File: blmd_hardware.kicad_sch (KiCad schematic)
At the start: 63 parts, among them J1 MR30PW-F, J2 control, J3 GND, J4 12V, J5 STLink-V3, Q1 RH6G040CH, Q2 RH6G040CH, Q3 RH6G040CH, Q4 RH6G040CH, Q5 RH6G040CH, Q6 RH6G040CH, SW1 reset, SW2 SW_DIP_x02, U1 A4939KLPTR-5-T, U10 STM32G431KBTx, U4 ISO7760FDBQR, U6 ACS711KEXLT-31AB, U7 ACS711KEXLT-31AB, U9 BD41041FJ-C

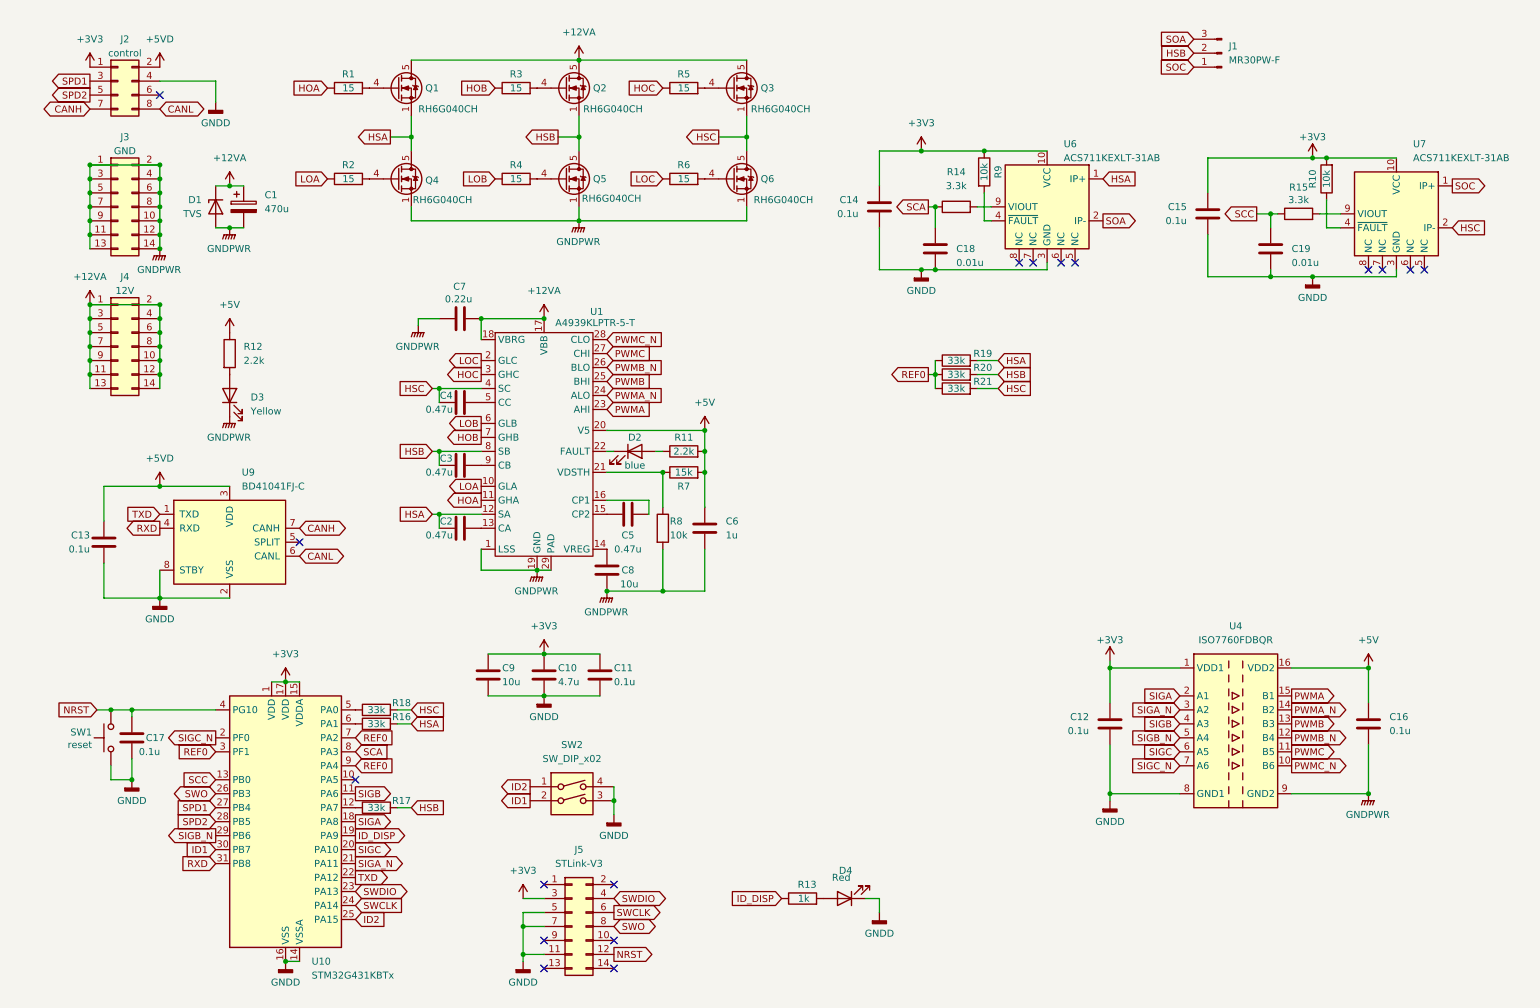
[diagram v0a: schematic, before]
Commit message: tmp : schemetic is all over except for can
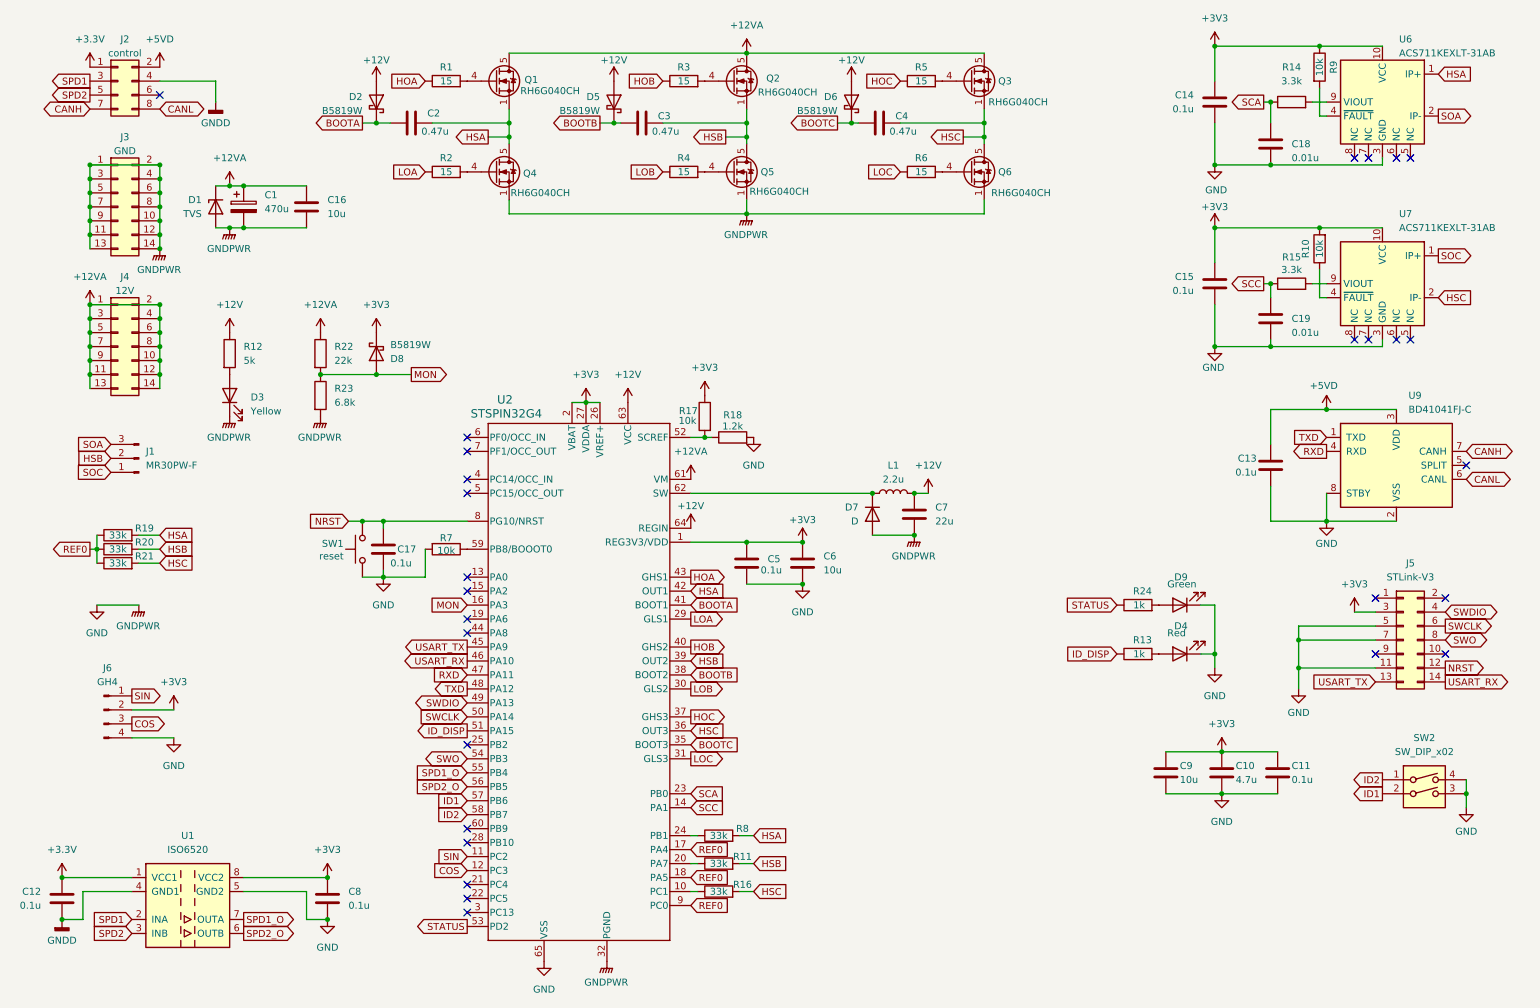
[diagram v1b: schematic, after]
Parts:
- removed D2: blue, LED_SMD:LED_0603_1608Metric_Pad1.05x0.95mm_HandSolder, symbol Device:LED
- removed U1: A4939KLPTR-5-T, Package_SO:HTSSOP-28-1EP_4.4x9.7mm_P0.65mm_EP2.75x6.2mm, symbol blmd:A4939KLPTR-5-T
- removed U10: STM32G431KBTx, Package_QFP:LQFP-32_7x7mm_P0.8mm, symbol MCU_ST_STM32G4:STM32G431KBTx
- removed U4: ISO7760FDBQR, Package_SO:SSOP-16_3.9x4.9mm_P0.635mm, symbol Isolator:Si8660BA-AS1
- added D2, D5, D6, D8: B5819W, Diode_SMD:D_SOD-123, symbol Device:D_Schottky
- added D7: D, symbol Device:D
- added D9: Green, LED_SMD:LED_0603_1608Metric_Pad1.05x0.95mm_HandSolder, symbol Device:LED
- added J6: GH4, symbol Connector:Conn_01x04_Pin
- added L1: 2.2u, symbol Device:L
- added R22: 22k, symbol Device:R
- added R23: 6.8k, symbol Device:R
- added R24: 1k, Resistor_SMD:R_0603_1608Metric_Pad0.98x0.95mm_HandSolder, symbol Device:R
- added U1: ISO6520, Package_SO:SOIC-8_3.9x4.9mm_P1.27mm, symbol Isolator:ISO7320C
- added U2: STSPIN32G4, QFN_IN32G4_STM, symbol blmd:STSPIN32G4
- C12, C2, C3, C4: footprint Capacitor_SMD:C_0603_1608Metric_Pad1.08x0.95mm_HandSolder -> (none)
- C16: value 0.1u -> 10u; footprint Capacitor_SMD:C_0603_1608Metric_Pad1.08x0.95mm_HandSolder -> (none)
- C5: value 0.47u -> 0.1u; footprint Capacitor_SMD:C_0603_1608Metric_Pad1.08x0.95mm_HandSolder -> (none)
- C6: value 1u -> 10u; footprint Capacitor_SMD:C_0603_1608Metric_Pad1.08x0.95mm_HandSolder -> (none)
- C7: value 0.22u -> 22u; footprint Capacitor_SMD:C_0603_1608Metric_Pad1.08x0.95mm_HandSolder -> (none)
- C8: value 10u -> 0.1u; footprint Capacitor_SMD:C_0603_1608Metric_Pad1.08x0.95mm_HandSolder -> (none)
- R11: value 2.2k -> 33k; footprint Resistor_SMD:R_0603_1608Metric_Pad0.98x0.95mm_HandSolder -> (none)
- R12: value 2.2k -> 5k
- R16: footprint Resistor_SMD:R_0603_1608Metric_Pad0.98x0.95mm_HandSolder -> (none)
- R17: value 33k -> 10k; footprint Resistor_SMD:R_0603_1608Metric_Pad0.98x0.95mm_HandSolder -> (none)
- R18: value 33k -> 1.2k; footprint Resistor_SMD:R_0603_1608Metric_Pad0.98x0.95mm_HandSolder -> (none)
- R7: value 15k -> 10k; footprint Resistor_SMD:R_0603_1608Metric_Pad0.98x0.95mm_HandSolder -> (none)
- R8: value 10k -> 33k; footprint Resistor_SMD:R_0603_1608Metric_Pad0.98x0.95mm_HandSolder -> (none)
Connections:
- net +12VA: now also C16.1, R22.1, U2.61 (VM); no longer C7.1
- net +3V3: now also C5.1, C6.1, C8.1, R17.1, D8.1 (K), J6.2 (Pin_2), U1.8 (VCC2), U2.1 (REG3V3/VDD), U2.2 (VBAT), U2.26 (VREF+), U2.27 (VDDA); no longer C12.1, J2.1 (Pin_1)
- net GNDD: now also U1.4 (GND1); no longer C10.2, C11.2, C13.2, C14.2, C15.2, C17.2, C18.2, C19.2, C9.2, D4.1 (K), J5.11 (Pin_11), J5.5 (Pin_5), J5.7 (Pin_7), SW1.1, SW2.3, SW2.4, U6.3 (GND), U7.3 (GND), U9.2 (VSS), U9.8 (STBY)
- net HOA: now also U2.43 (GHS1)
- net HOB: now also U2.40 (GHS2)
- net HOC: now also U2.37 (GHS3)
- net HSA: now also R8.2, U2.42 (OUT1); no longer R16.2
- net HSB: now also C3.2, R11.2, U2.39 (OUT2); no longer C3.1, R17.2
- net HSC: now also C4.2, R16.2, U2.36 (OUT3); no longer C4.1, R18.2
- net ID1: now also U2.57 (PB6)
- net ID2: now also U2.58 (PB7)
- net ID_DISP: now also U2.51 (PA15)
- net LOA: now also U2.29 (GLS1)
- net LOB: now also U2.30 (GLS2)
- net LOC: now also U2.31 (GLS3)
- net NRST: now also U2.8 (PG10/NRST)
- net REF0: now also U2.17 (PA4), U2.18 (PA5), U2.9 (PC0)
- net RXD: now also U2.47 (PA11)
- net SCA: now also U2.23 (PB0)
- net SCC: now also U2.14 (PA1)
- net SPD1: now also U1.2 (INA)
- net SPD2: now also U1.3 (INB)
- net SWCLK: now also U2.50 (PA14)
- net SWDIO: now also U2.49 (PA13)
- net SWO: now also U2.54 (PB3)
- net TXD: now also U2.48 (PA12)
- net at R18.1: now also R17.2, U2.52 (SCREF)
- net at R16.1: now also U2.10 (PC1)
- net GND: now reaches C8.2
- net GND: now also C1.2, C10.2, C11.2, C13.2, C14.2, C15.2, C16.2, C17.2, C18.2, C19.2, C5.2, C6.2, C7.2, C9.2, D1.2 (A), D3.1 (K), D4.1 (K), J3.1 (Pin_1), J3.10 (Pin_10), J3.11 (Pin_11), J3.12 (Pin_12), J3.13 (Pin_13), J3.14 (Pin_14), J3.2 (Pin_2), J3.3 (Pin_3), J3.4 (Pin_4), J3.5 (Pin_5), J3.6 (Pin_6), J3.7 (Pin_7), J3.8 (Pin_8), J3.9 (Pin_9), J5.11 (Pin_11), J5.5 (Pin_5), J5.7 (Pin_7), Q4.1 (S), Q4.2 (S), Q4.3 (S), Q5.1 (S), Q5.2 (S), Q5.3 (S), Q6.1 (S), Q6.2 (S), Q6.3 (S), R18.2, R7.2, SW1.1, SW2.3, SW2.4, U6.3 (GND), U7.3 (GND), U9.2 (VSS), U9.8 (STBY), D7.2 (A), D9.1 (K), J6.4 (Pin_4), R23.2, U1.5 (GND2), U2.32 (PGND), U2.65 (VSS)
- net BOOTA: now reaches C2.2
- net BOOTA: now also D2.1 (K), U2.41 (BOOT1)
- net at R8.1: now also U2.24 (PB1); no longer R7.1
- net at R11.1: now also U2.20 (PA7)
- net USART_TX: now reaches J5.13 (Pin_13)
- net USART_TX: now also U2.45 (PA9)
- net USART_RX: now reaches J5.14 (Pin_14)
- net USART_RX: now also U2.46 (PA10)
- removed net +5V: C16.1, C6.1, R11.2, R12.1, R7.2
- removed net GNDPWR: C1.2, C16.2, C6.2, C7.2, C8.1, D1.2 (A), D3.1 (K), J3.1 (Pin_1), J3.10 (Pin_10), J3.11 (Pin_11), J3.12 (Pin_12), J3.13 (Pin_13), J3.14 (Pin_14), J3.2 (Pin_2), J3.3 (Pin_3), J3.4 (Pin_4), J3.5 (Pin_5), J3.6 (Pin_6), J3.7 (Pin_7), J3.8 (Pin_8), J3.9 (Pin_9), Q4.1 (S), Q4.2 (S), Q4.3 (S), Q5.1 (S), Q5.2 (S), Q5.3 (S), Q6.1 (S), Q6.2 (S), Q6.3 (S), R8.2
- new net: D9.2 (A), R24.2
- new net: D7.1 (K), L1.1, U2.62 (SW)
- new net: U2.33 (NC), U2.34 (NC)
- new net: R7.1, U2.59 (PB8/BOOOT0)
- new net +12V: C7.1, D2.2 (A), D5.2 (A), D6.2 (A), L1.2, R12.1, U2.63 (VCC), U2.64 (REGIN)
- new net +3.3V: C12.1, J2.1 (Pin_1), U1.1 (VCC1)
- new net BOOTB: C3.1, D5.1 (K), U2.38 (BOOT2)
- new net BOOTC: C4.1, D6.1 (K), U2.35 (BOOT3)
- new net COS: J6.3 (Pin_3), U2.12 (PC3)
- new net MON: D8.2 (A), R22.2, R23.1, U2.16 (PA3)
- new net SIN: J6.1 (Pin_1), U2.11 (PC2)
- new net SPD1_O: U1.7 (OUTA), U2.55 (PB4)
- new net SPD2_O: U1.6 (OUTB), U2.56 (PB5)
- new net STATUS: R24.1, U2.53 (PD2)
- no-connect marks 17 -> 28
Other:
- moved on the sheet: C10, C11, C13, C14, C15, C17, C18, C19, C9, D4, J1, J5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

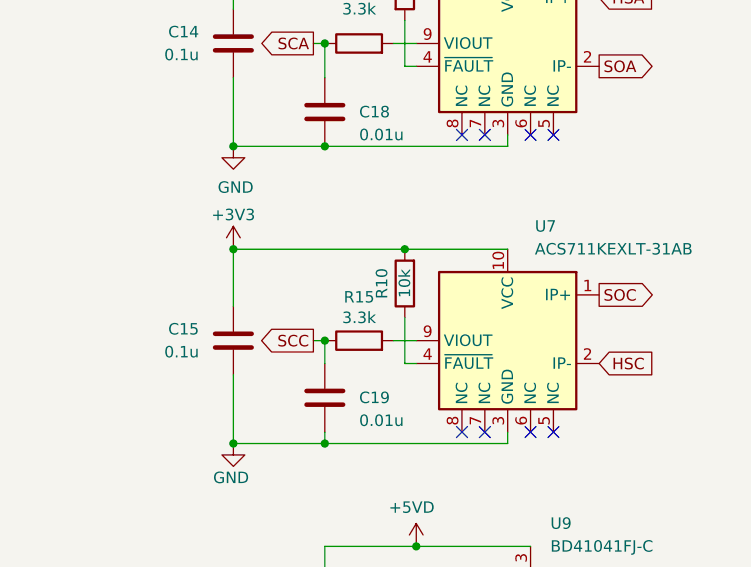
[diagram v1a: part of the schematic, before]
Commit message: tmp : backup commit
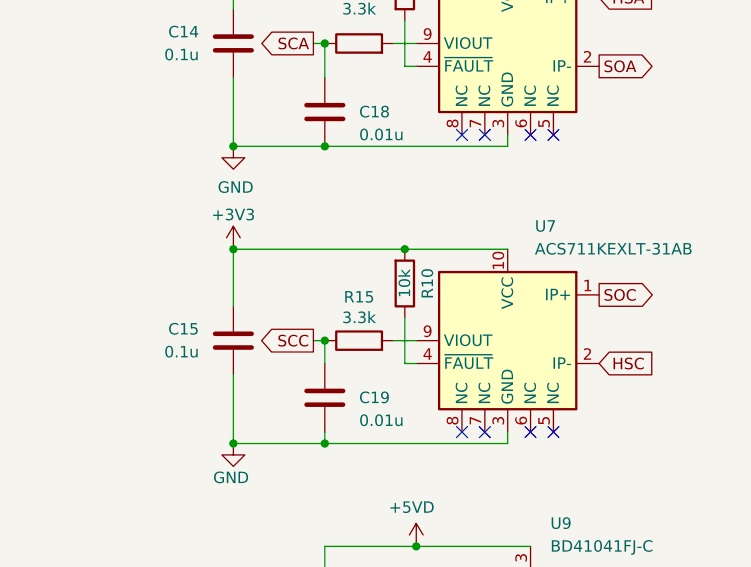
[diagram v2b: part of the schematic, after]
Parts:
- U2: footprint QFN_IN32G4_STM -> blmd_hardware:QFN_IN32G4_STM
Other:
- moved on the sheet: R10
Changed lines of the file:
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@@
 	(symbol
 		(lib_id "Device:R")
-		(at 248.92 57.15 180)
+		(at 248.92 57.15 0)
+		(mirror x)
 		(unit 1)
 		(exclude_from_sim no)
@@
 		(dnp no)
 		(property "Reference" "R10"
-			(at 246.38 57.15 90)
+			(at 251.46 57.15 90)
 			(effects
 				(font
@@
 		)
 		(property "Footprint" "Resistor_SMD:R_0603_1608Metric_Pad0.98x0.95mm_HandSolder"
-			(at 250.698 57.15 90)
+			(at 247.142 57.15 90)
 			(effects
 				(font
@@
 			)
 		)
-		(property "Footprint" "QFN_IN32G4_STM"
+		(property "Footprint" "blmd_hardware:QFN_IN32G4_STM"
 			(at 90.17 93.98 0)
 			(effects
